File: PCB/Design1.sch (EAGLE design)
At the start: 38 parts, among them J1 FTDI_DEVICE, U1 ATMEGA2560AU

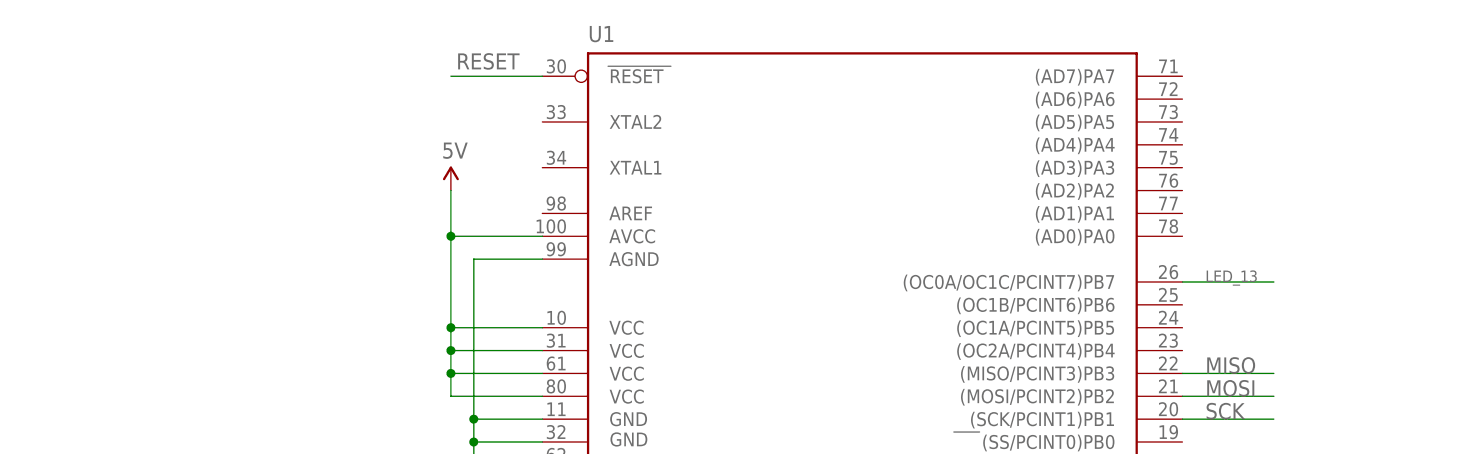
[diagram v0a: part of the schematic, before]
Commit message: meh
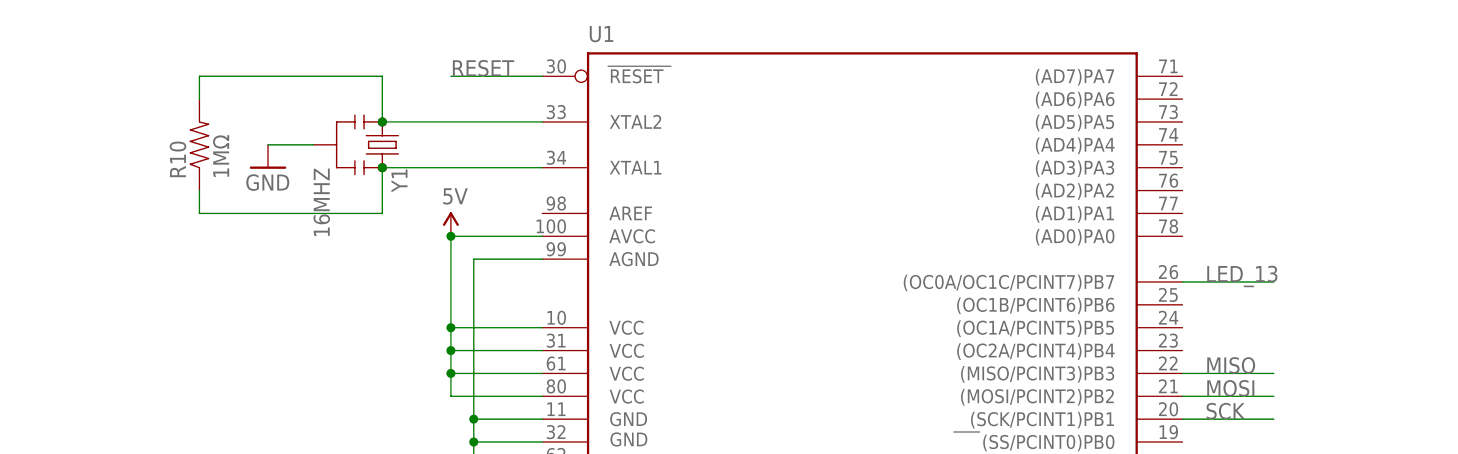
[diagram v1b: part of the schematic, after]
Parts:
- added R10: 1MΩ, SparkFun-Resistors:RESISTOR1206
- added Y1: 16MHZ, SparkFun-FreqCtrl:RESONATOR16MHZ
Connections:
- net N$8 renamed VIN_RECTIFIED
- new net XTAL1: R10.1, U1.XTAL1, Y1.3
- new net XTAL2: R10.2, U1.XTAL2, Y1.1
- net GND: now also Y1.2
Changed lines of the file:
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@@
 <part name="U3" library="SparkFun-PowerIC" deviceset="V_REG_LM1117" device="SOT223"/>
 <part name="C7" library="SparkFun-Capacitors" deviceset="CAP_POL" device="PTH1" value="470uF"/>
+<part name="Y1" library="SparkFun-FreqCtrl" deviceset="RESONATOR" device="16MHZ" value="16MHZ"/>
+<part name="R10" library="SparkFun-Resistors" deviceset="RESISTOR" device="1206" value="1MΩ"/>
+<part name="GND8" library="SparkFun-Aesthetics" deviceset="GND" device=""/>
 </parts>
 <sheets>
@@
 <instance part="POWER" gate="G$1" x="5.08" y="33.02"/>
 <instance part="SERIAL" gate="G$1" x="256.54" y="73.66"/>
-<instance part="SUPPLY1" gate="G$1" x="60.96" y="205.74"/>
+<instance part="SUPPLY1" gate="G$1" x="60.96" y="200.66"/>
 <instance part="SUPPLY3" gate="G$1" x="238.76" y="25.4"/>
 <instance part="SUPPLY5" gate="G$1" x="111.76" y="43.18"/>
@@
 <instance part="U3" gate="G$1" x="63.5" y="20.32" rot="MR180"/>
 <instance part="C7" gate="G$1" x="81.28" y="35.56"/>
+<instance part="Y1" gate="G$1" x="53.34" y="210.82" rot="R270"/>
+<instance part="R10" gate="G$1" x="33.02" y="210.82" rot="R90"/>
+<instance part="GND8" gate="1" x="40.64" y="208.28"/>
 </instances>
 <busses>
@@
 <junction x="274.32" y="177.8"/>
 </segment>
+<segment>
+<pinref part="Y1" gate="G$1" pin="2"/>
+<wire x1="45.72" y1="210.82" x2="40.64" y2="210.82" width="0.1524" layer="91"/>
+<pinref part="GND8" gate="1" pin="GND"/>
+</segment>
 </net>
 <net name="RESET" class="0">
@@
 <pinref part="U1" gate="1" pin="RESET"/>
 <wire x1="71.12" y1="218.44" x2="60.96" y2="218.44" width="0.1524" layer="91"/>
-<label x="68.58" y="220.98" size="1.778" layer="95" rot="R180"/>
+<label x="60.96" y="218.44" size="1.778" layer="95"/>
 </segment>
 </net>
@@
 <pinref part="U1" gate="1" pin="(OC0A/OC1C/PCINT7)PB7"/>
 <wire x1="142.24" y1="195.58" x2="152.4" y2="195.58" width="0.1524" layer="91"/>
-<label x="144.78" y="195.58" size="1.27" layer="95"/>
+<label x="144.78" y="195.58" size="1.778" layer="95"/>
 </segment>
 </net>
@@
 <wire x1="71.12" y1="200.66" x2="60.96" y2="200.66" width="0.1524" layer="91"/>
 <pinref part="SUPPLY1" gate="G$1" pin="5V"/>
-<wire x1="60.96" y1="205.74" x2="60.96" y2="200.66" width="0.1524" layer="91"/>
 <junction x="60.96" y="200.66"/>
 </segment>
@@
 </segment>
 </net>
-<net name="N$8" class="0">
+<net name="VIN_RECTIFIED" class="0">
 <segment>
 <pinref part="D2" gate="G$1" pin="C"/>
@@
 </segment>
 </net>
+<net name="XTAL2" class="0">
+<segment>
+<pinref part="Y1" gate="G$1" pin="1"/>
+<pinref part="U1" gate="1" pin="XTAL2"/>
+<wire x1="71.12" y1="213.36" x2="53.34" y2="213.36" width="0.1524" layer="91"/>
+<wire x1="53.34" y1="213.36" x2="53.34" y2="218.44" width="0.1524" layer="91"/>
+<junction x="53.34" y="213.36"/>
+<pinref part="R10" gate="G$1" pin="2"/>
+<wire x1="53.34" y1="218.44" x2="33.02" y2="218.44" width="0.1524" layer="91"/>
+<wire x1="33.02" y1="218.44" x2="33.02" y2="215.9" width="0.1524" layer="91"/>
+</segment>
+</net>
+<net name="XTAL1" class="0">
+<segment>
+<pinref part="Y1" gate="G$1" pin="3"/>
+<pinref part="U1" gate="1" pin="XTAL1"/>
+<wire x1="71.12" y1="208.28" x2="53.34" y2="208.28" width="0.1524" layer="91"/>
+<wire x1="53.34" y1="208.28" x2="53.34" y2="203.2" width="0.1524" layer="91"/>
+<junction x="53.34" y="208.28"/>
+<pinref part="R10" gate="G$1" pin="1"/>
+<wire x1="53.34" y1="203.2" x2="33.02" y2="203.2" width="0.1524" layer="91"/>
+<wire x1="33.02" y1="203.2" x2="33.02" y2="205.74" width="0.1524" layer="91"/>
+</segment>
+</net>
